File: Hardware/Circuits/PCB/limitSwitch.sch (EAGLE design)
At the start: 9 parts

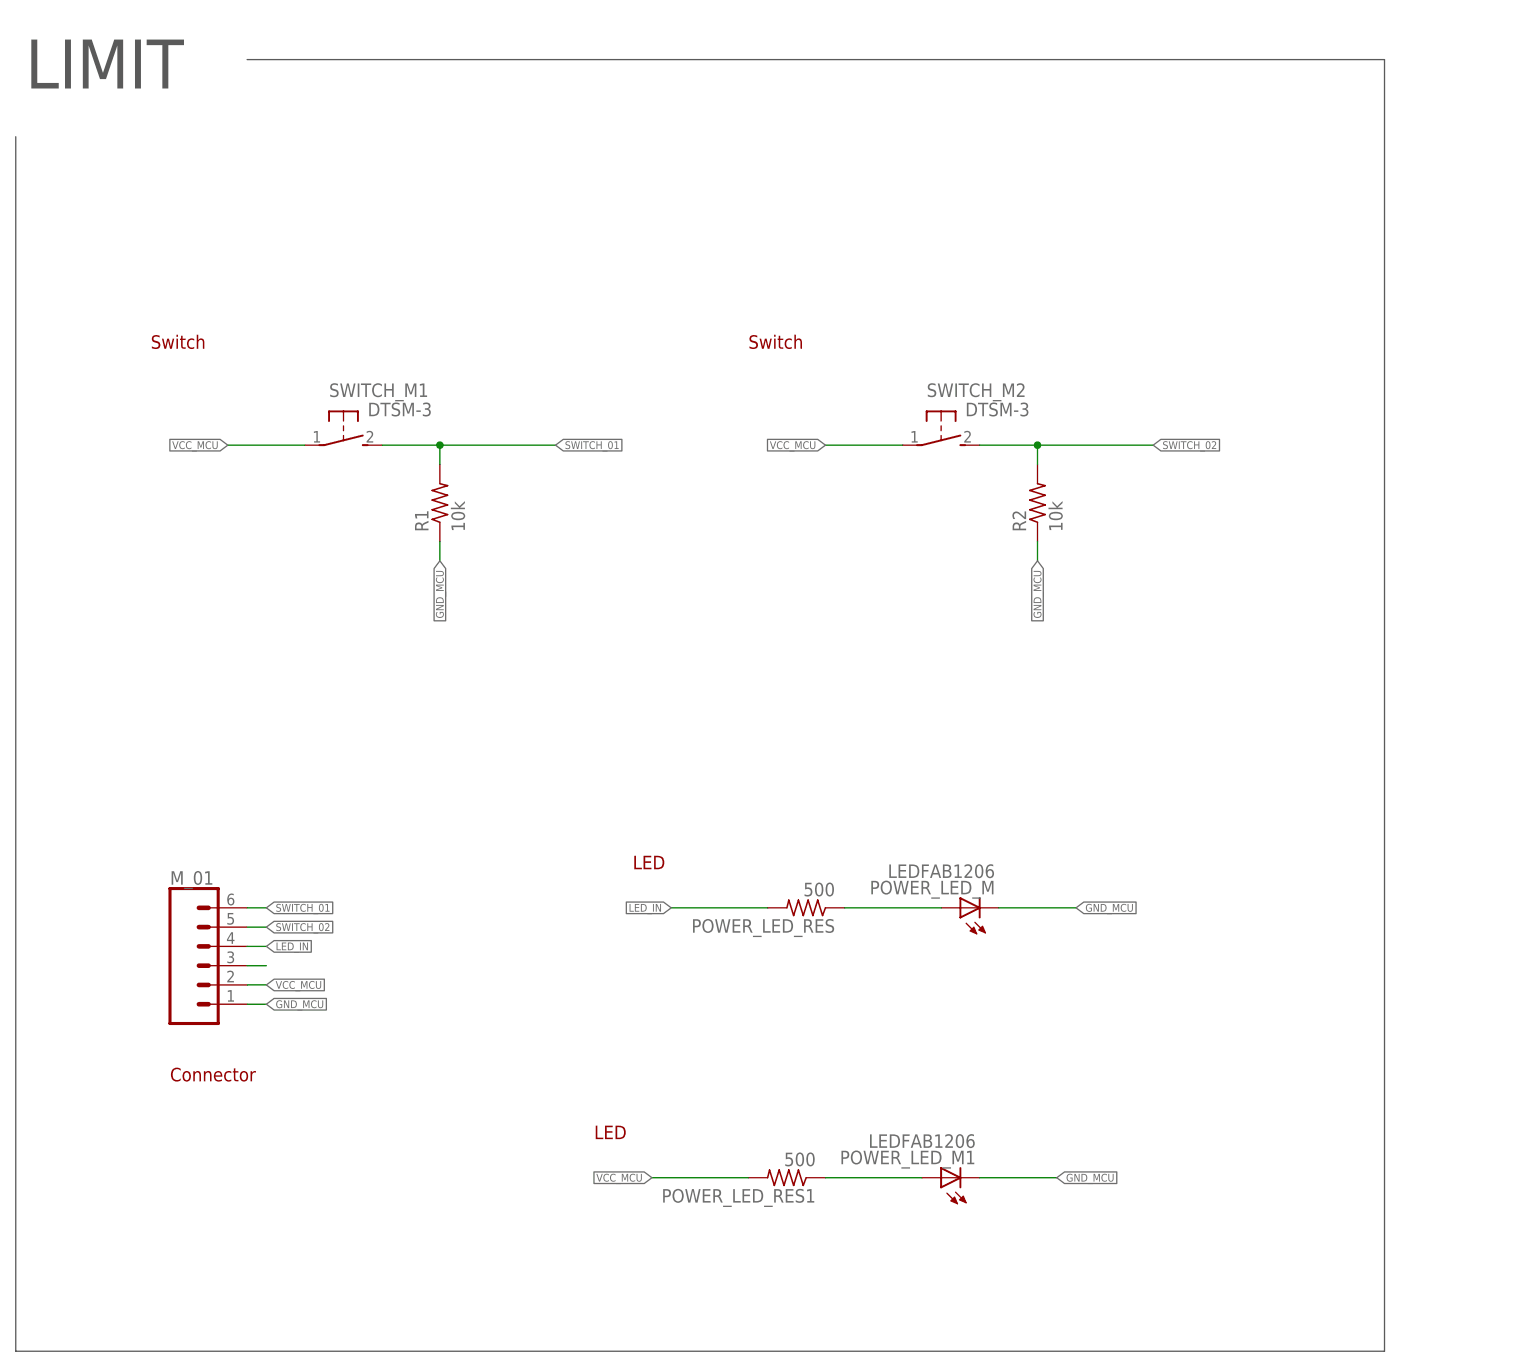
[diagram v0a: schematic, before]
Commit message: circuits
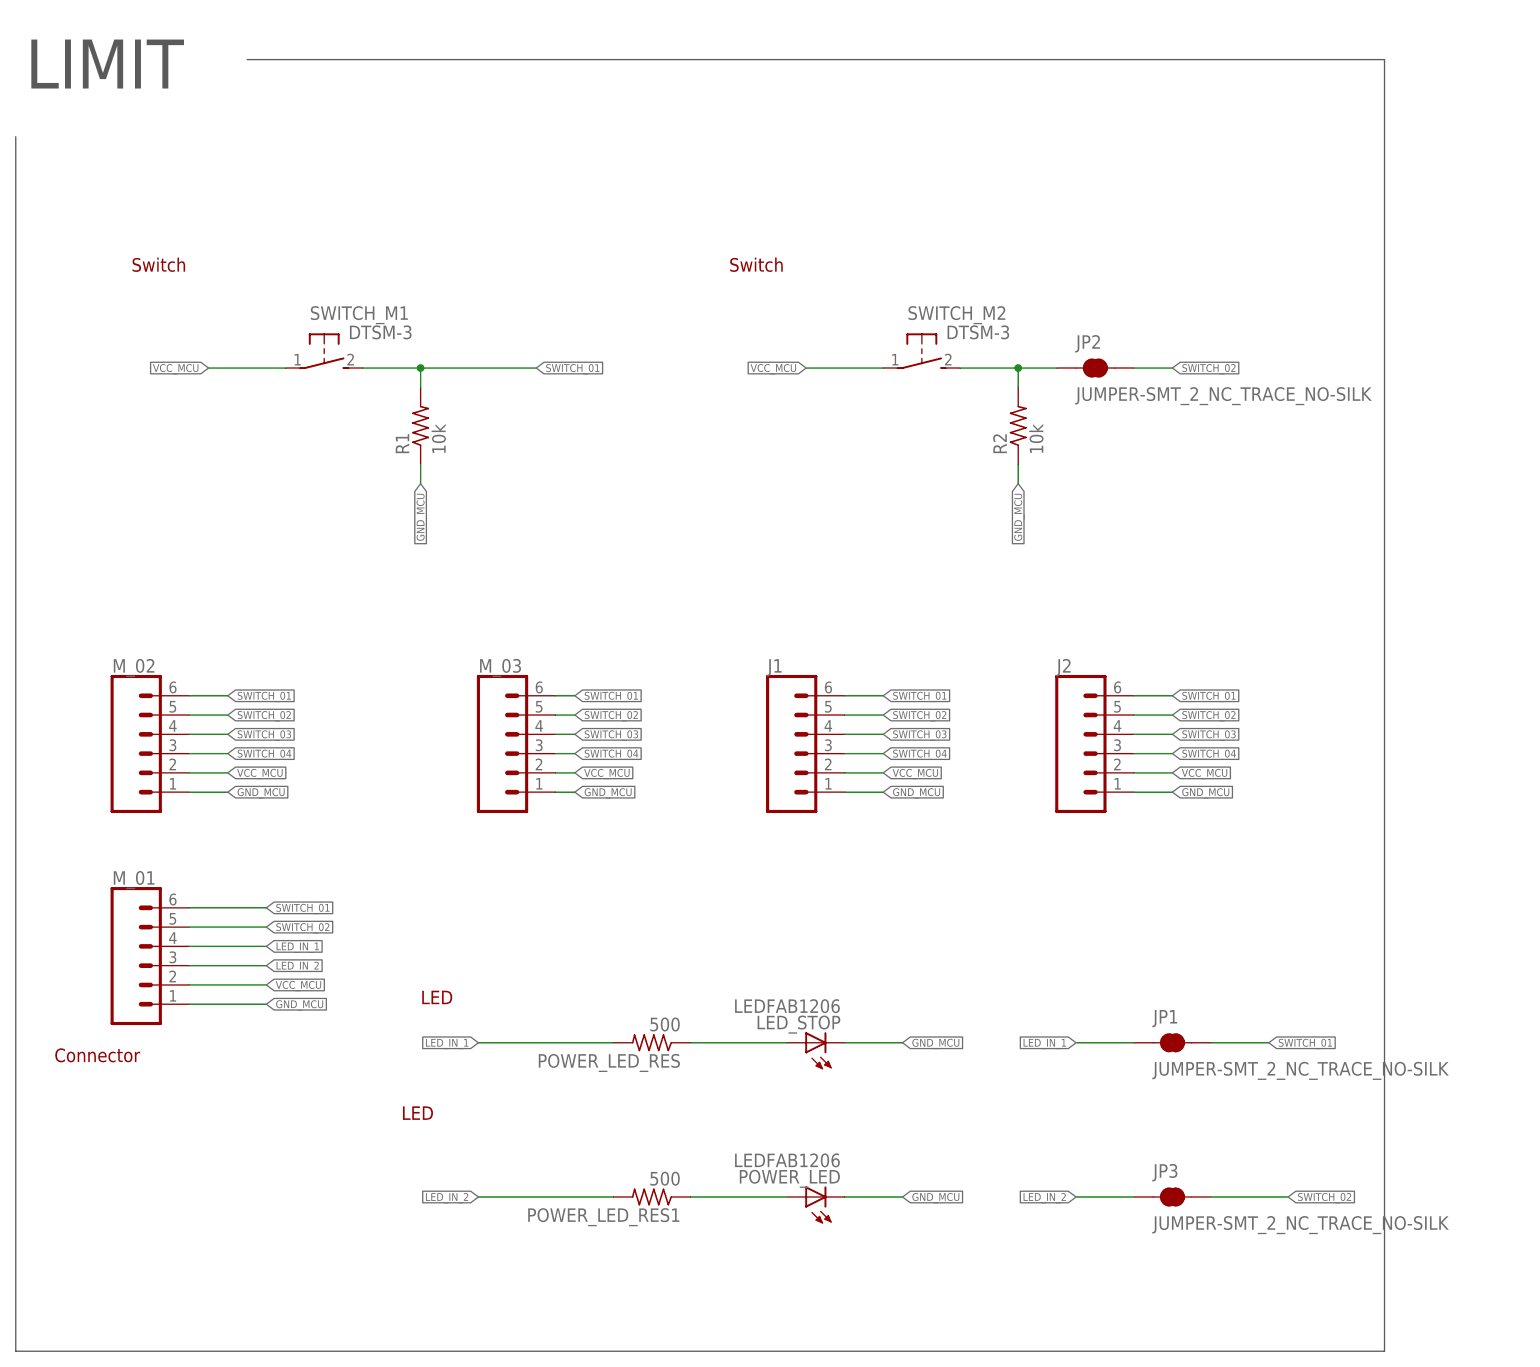
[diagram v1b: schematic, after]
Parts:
- removed POWER_LED_M, POWER_LED_M1: LEDFAB1206, fab:LEDFAB1206
- added J1, J2: (no value), SparkFun-Connectors:CONN_06NO_SILK_FEMALE_PTH
- added JP1, JP2, JP3: JUMPER-SMT_2_NC_TRACE_NO-SILK, SparkFun-Jumpers:JUMPER-SMT_2_NC_TRACE_NO-SILK
- added LED_STOP, POWER_LED: LEDFAB1206, fab:LEDFAB1206
- added M_02, M_03: (no value), SparkFun-Connectors:CONN_06SMD-1MM
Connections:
- removed net LED_IN: M_01.4, POWER_LED_RES.2
- removed net NEO_PIXEL: M_01.3
- new net LED_IN_1: JP1.1, M_01.4, POWER_LED_RES.2
- new net LED_IN_2: JP3.1, M_01.3, POWER_LED_RES1.2
- new net N$2: JP2.1, R2.2, SWITCH_M2.2
- new net SWITCH_03: J1.4, J2.4, M_02.4, M_03.4
- new net SWITCH_04: J1.3, J2.3, M_02.3, M_03.3
- net GND_MCU: now also J1.1, J2.1, LED_STOP.C, M_02.1, M_03.1, POWER_LED.C; no longer POWER_LED_M.C, POWER_LED_M1.C
- net N$1: now also POWER_LED.A; no longer POWER_LED_M1.A
- net N$11: now also LED_STOP.A; no longer POWER_LED_M.A
- net SWITCH_01: now also J1.6, J2.6, JP1.2, M_02.6, M_03.6
- net SWITCH_02: now also J1.5, J2.5, JP2.2, JP3.2, M_02.5, M_03.5; no longer R2.2, SWITCH_M2.2
- net VCC_MCU: now also J1.2, J2.2, M_02.2, M_03.2; no longer POWER_LED_RES1.2
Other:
- moved on the sheet: M_01, POWER_LED_RES, POWER_LED_RES1, R1, R2, SWITCH_M1, SWITCH_M2
